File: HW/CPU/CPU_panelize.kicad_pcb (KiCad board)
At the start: 2 copper layers, 215 x 212 mm, 272 parts, among them J1 I2C, J2 SBW, J3 PWR, U1 CONRAD_USB_UART, U2 MSP430G2452, X1 XTAL

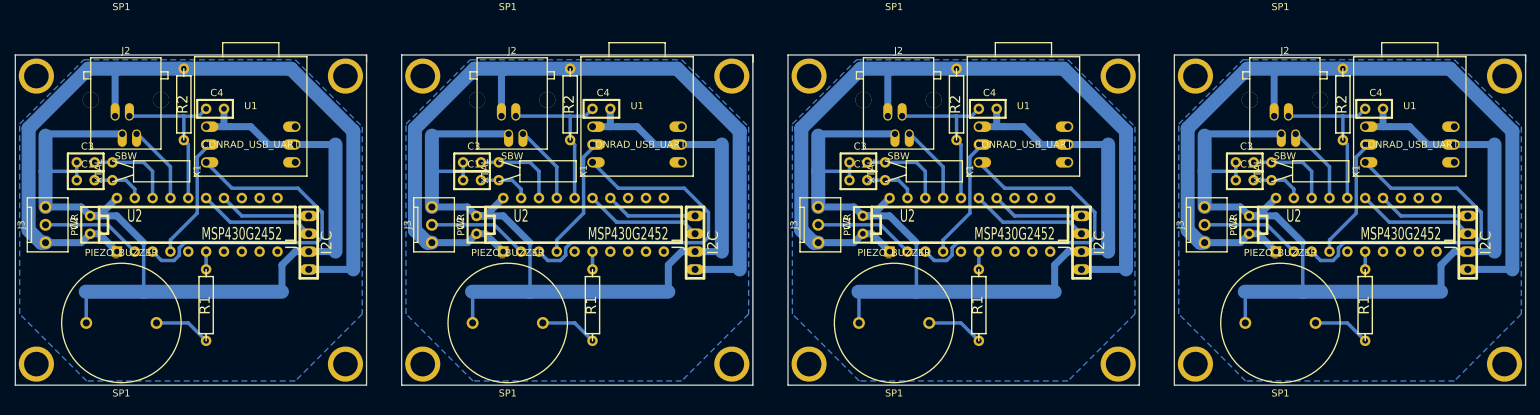
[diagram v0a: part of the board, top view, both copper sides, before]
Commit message: x
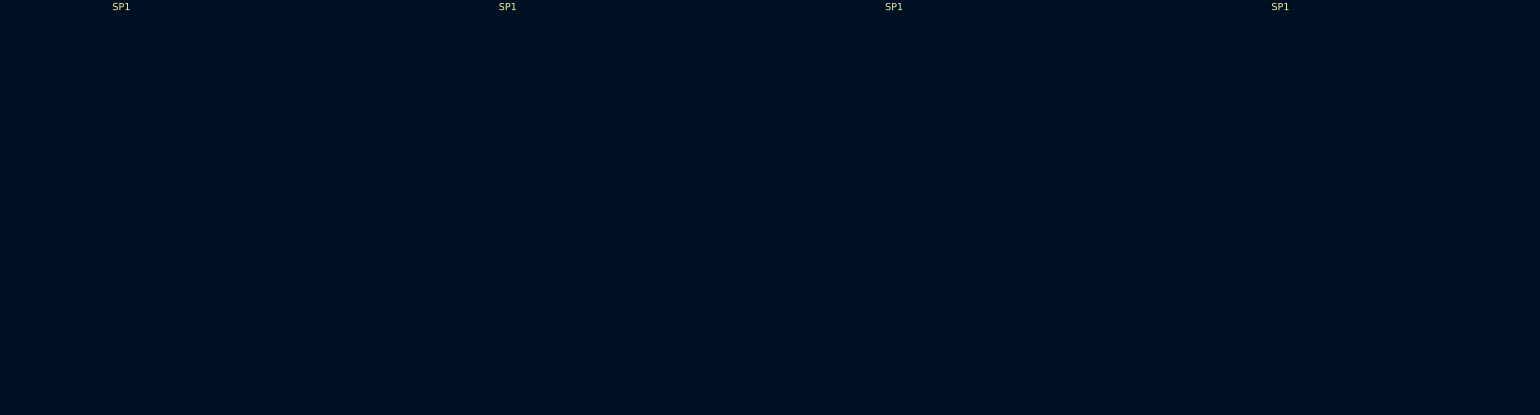
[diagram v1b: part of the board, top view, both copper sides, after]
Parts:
- removed the C1 at (140.0, 202.8)
- removed the C1 at (195.0, 202.8)
- removed the C1 at (85.0, 202.8)
- removed the C1 at (30.0, 202.8)
- removed the C2 at (140.7, 209.2)
- removed the C2 at (195.7, 209.2)
- removed the C2 at (85.7, 209.2)
- removed the C2 at (30.7, 209.2)
- removed the C3 at (140.0, 200.3)
- removed the C3 at (195.0, 200.3)
- removed the C3 at (85.0, 200.3)
- removed the C3 at (30.0, 200.3)
- removed the C4 at (158.4, 192.7)
- removed the C4 at (213.4, 192.7)
- removed the C4 at (103.4, 192.7)
- removed the C4 at (48.4, 192.7)
- removed the J1 at (171.8, 211.7)
- removed the J1 at (226.8, 211.7)
- removed the J1 at (116.8, 211.7)
- removed the J1 at (61.8, 211.7)
- removed the J2 at (145.7, 191.4)
- removed the J2 at (200.7, 191.4)
- removed the J2 at (90.7, 191.4)
- removed the J2 at (35.7, 191.4)
- removed the J3 at (134.3, 209.2)
- removed the J3 at (189.3, 209.2)
- removed the J3 at (79.3, 209.2)
- removed the J3 at (24.3, 209.2)
- removed the MNT_HOLE_3.5S at (133.0, 188.0)
- removed the MNT_HOLE_3.5S at (133.0, 229.0)
- removed the MNT_HOLE_3.5S at (177.0, 229.0)
- removed the MNT_HOLE_3.5S at (177.0, 188.0)
- removed the MNT_HOLE_3.5S at (232.0, 188.0)
- removed the MNT_HOLE_3.5S at (232.0, 229.0)
- removed the MNT_HOLE_3.5S at (188.0, 229.0)
- removed the MNT_HOLE_3.5S at (188.0, 188.0)
- removed the MNT_HOLE_3.5S at (78.0, 188.0)
- removed the MNT_HOLE_3.5S at (78.0, 229.0)
- removed the MNT_HOLE_3.5S at (122.0, 229.0)
- removed the MNT_HOLE_3.5S at (122.0, 188.0)
- removed the MNT_HOLE_3.5S at (67.0, 188.0)
- removed the MNT_HOLE_3.5S at (67.0, 229.0)
- removed the MNT_HOLE_3.5S at (23.0, 229.0)
- removed the MNT_HOLE_3.5S at (23.0, 188.0)
- removed the R1 at (157.2, 220.6)
- removed the R1 at (212.2, 220.6)
- removed the R1 at (102.2, 220.6)
- removed the R1 at (47.2, 220.6)
- removed the R2 at (154.0, 192.0)
- removed the R2 at (209.0, 192.0)
- removed the R2 at (99.0, 192.0)
- removed the R2 at (44.0, 192.0)
- removed the SP1 at (145.1, 223.1)
- removed the SP1 at (200.1, 223.1)
- removed the SP1 at (90.1, 223.1)
- removed the SP1 at (35.1, 223.1)
- removed the U1 at (163.5, 197.7)
- removed the U1 at (218.5, 197.7)
- removed the U1 at (108.5, 197.7)
- removed the U1 at (53.5, 197.7)
- removed the U2 at (155.9, 209.2)
- removed the U2 at (210.9, 209.2)
- removed the U2 at (100.9, 209.2)
- removed the U2 at (45.9, 209.2)
- removed the X1 at (143.8, 201.6)
- removed the X1 at (198.8, 201.6)
- removed the X1 at (88.8, 201.6)
- removed the X1 at (33.8, 201.6)
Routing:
- net GND: track 2210.5 -> 1657.9 mm
- net VCC: track 1853.6 -> 1390.2 mm
- net N-000009: track 794.1 -> 595.6 mm
- net N-0000023: track 372.4 -> 279.3 mm
- net N-0000012: track 289.0 -> 216.8 mm
- net N-000007: track 267.3 -> 200.5 mm
- net N-000001: track 228.5 -> 171.3 mm
- net N-000008: track 209.9 -> 157.4 mm
- net N-0000014: track 201.5 -> 151.1 mm
- net N-000002: track 182.3 -> 136.8 mm
- net N-000004: track 129.9 -> 97.4 mm
- net N-0000013: track 120.2 -> 90.1 mm
- net N-000005: track 40.6 -> 30.5 mm
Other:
- board size 215 x 212 mm -> 215 x 157 mm
